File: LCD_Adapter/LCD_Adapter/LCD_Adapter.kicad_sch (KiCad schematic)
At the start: 2 parts, among them J1 2-1734248-0, J2 FH12-30S-0.5SH_55_

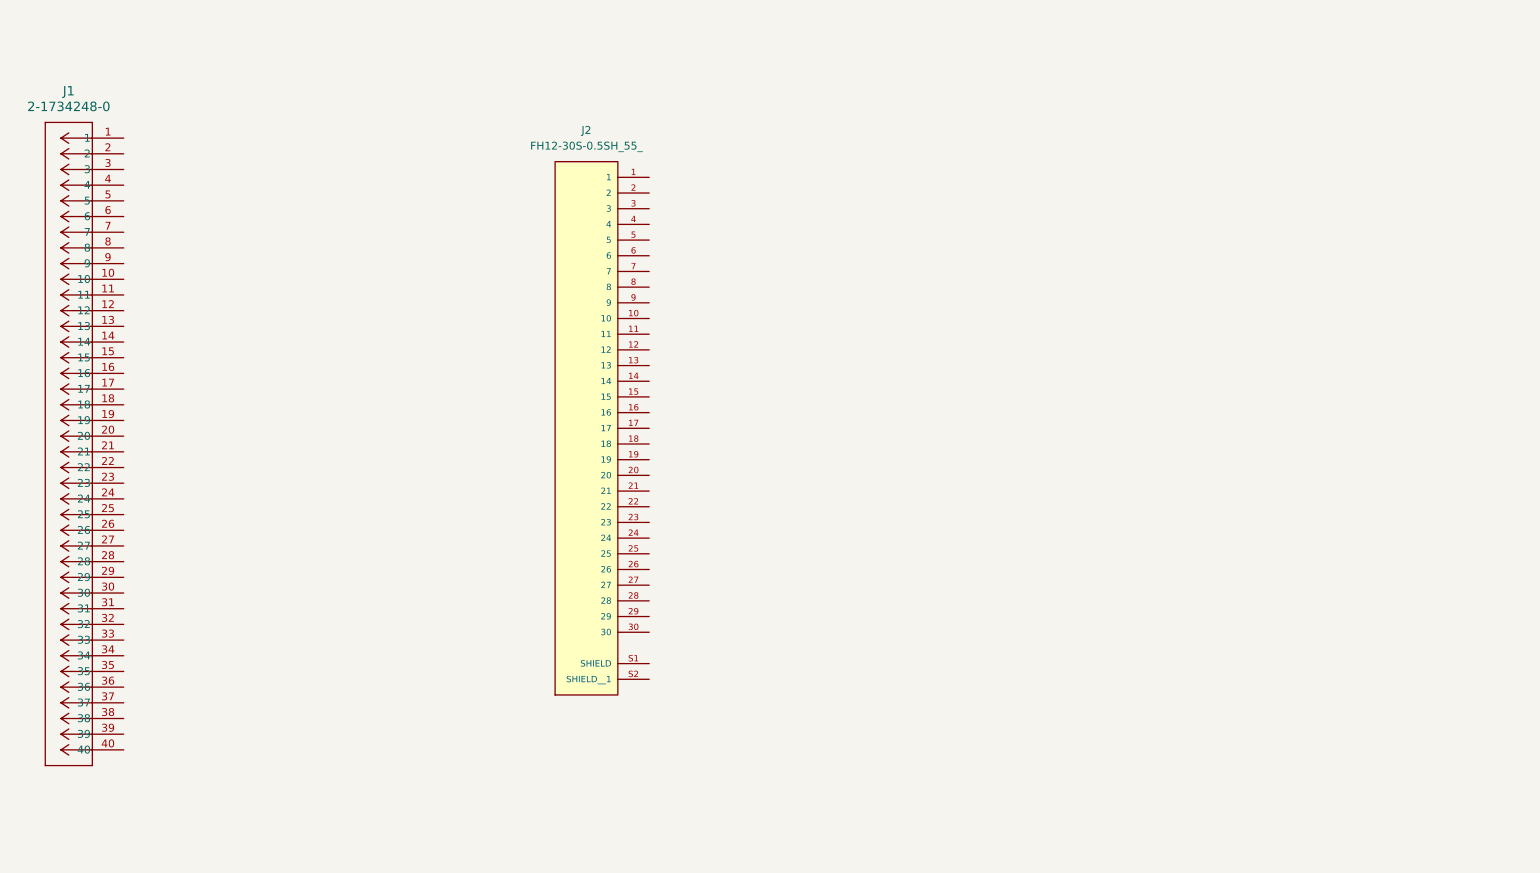
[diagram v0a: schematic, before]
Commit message: PSB_ADAPTER UPDATE
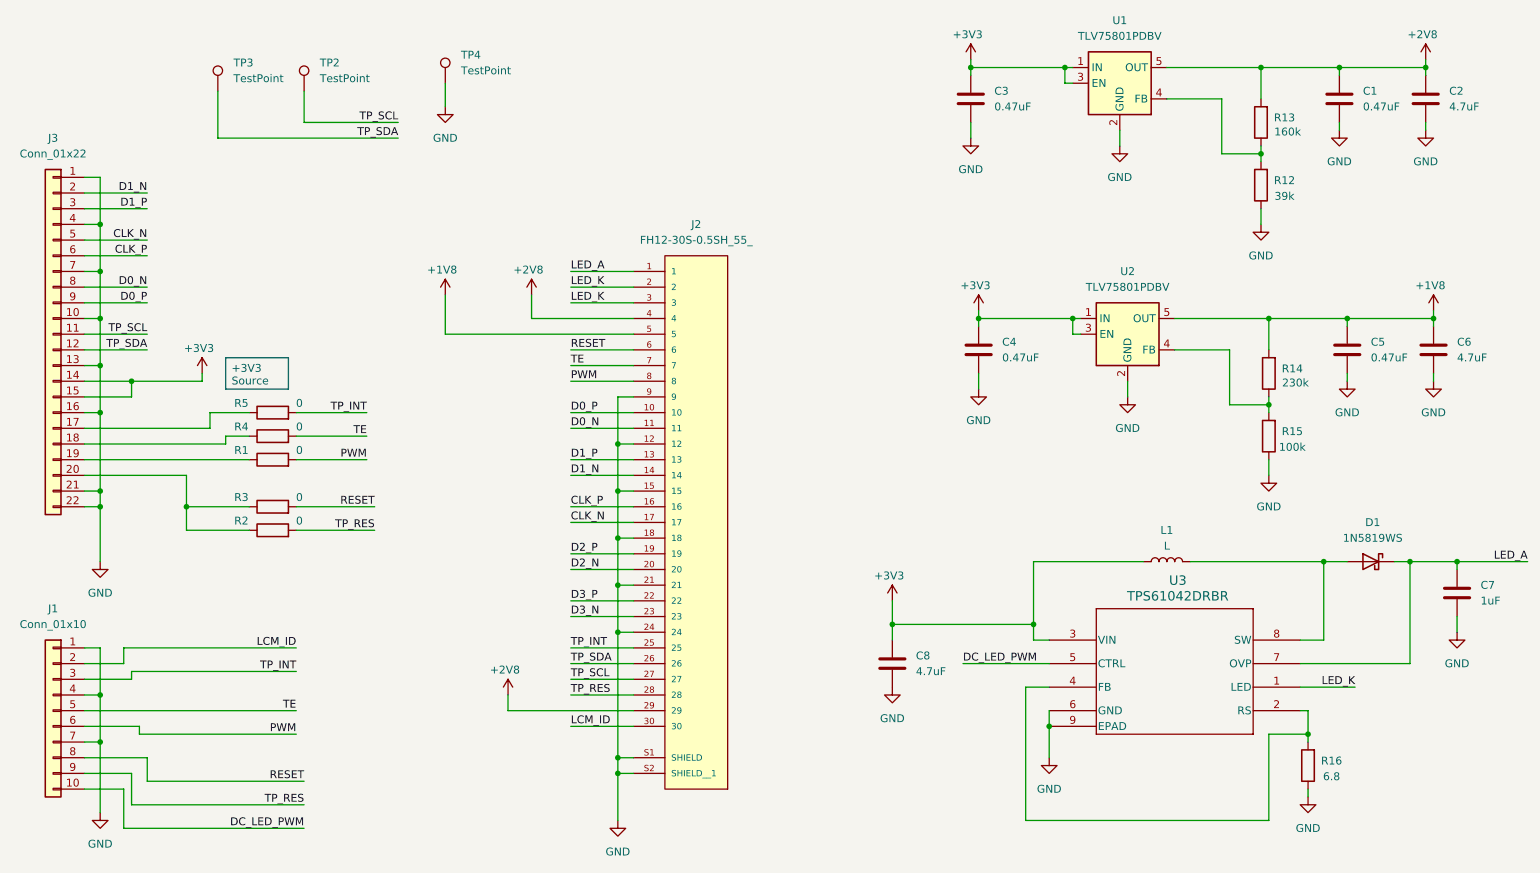
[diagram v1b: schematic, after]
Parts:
- removed J1: 2-1734248-0, lib:2-1734248-0, symbol 2-1734248-0:2-1734248-0
- added C1, C3, C4, C5: 0.47uF, Capacitor_SMD:C_0603_1608Metric, symbol Device:C
- added C2, C6, C8: 4.7uF, Capacitor_SMD:C_0603_1608Metric, symbol Device:C
- added C7: 1uF, Capacitor_SMD:C_0603_1608Metric, symbol Device:C
- added D1: 1N5819WS, Diode_SMD:D_SOD-323, symbol Diode:1N5819WS
- added J1: Conn_01x10, Connector_PinHeader_2.54mm:PinHeader_1x10_P2.54mm_Vertical, symbol Connector_Generic:Conn_01x10
- added J3: Conn_01x22, lib:FC-10A20P11H20, symbol Connector_Generic:Conn_01x22
- added L1: L, Inductor_SMD:L_1210_3225Metric, symbol Device:L
- added R1, R2, R3, R4, R5: 0, Resistor_SMD:R_0603_1608Metric, symbol Device:R
- added R12: 39k, Resistor_SMD:R_0603_1608Metric, symbol Device:R
- added R13: 160k, Resistor_SMD:R_0603_1608Metric, symbol Device:R
- added R14: 230k, Resistor_SMD:R_0603_1608Metric, symbol Device:R
- added R15: 100k, Resistor_SMD:R_0603_1608Metric, symbol Device:R
- added R16: 6.8, Resistor_SMD:R_0603_1608Metric, symbol Device:R
- added TP2, TP3, TP4: TestPoint, TestPoint:TestPoint_Pad_D1.0mm, symbol Connector:TestPoint
- added U1, U2: TLV75801PDBV, Package_TO_SOT_SMD:SOT-23-5, symbol Regulator_Linear:TLV75801PDBV
- added U3: TPS61042DRBR, lib:DRB8_1P75X1P5, symbol TPS61042:TPS61042DRBR
- J2: footprint FH12-30S-0.5SH_55_:HIROSE_FH12-30S-0.5SH_55_ -> lib:HIROSE_FH12-30S-0.5SH_55_
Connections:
- net  LED_A: now reaches J2.1
- net  LED_A: now also C7.1, D1.1 (K), U3.7 (OVP)
- net D0_P: now reaches J2.10
- net D0_P: now also J3.9 (Pin_9)
- net D0_N: now reaches J2.11
- net D0_N: now also J3.8 (Pin_8)
- net GND: now reaches J2.12
- net GND: now also J2.15, J2.18, J2.21, J2.24, J2.9, J2.S1 (SHIELD), J2.S2 (SHIELD__1), C1.2, C2.2, C3.2, C4.2, C5.2, C6.2, C7.2, C8.2, J1.1 (Pin_1), J1.4 (Pin_4), J1.7 (Pin_7), J3.1 (Pin_1), J3.10 (Pin_10), J3.13 (Pin_13), J3.16 (Pin_16), J3.21 (Pin_21), J3.22 (Pin_22), J3.4 (Pin_4), J3.7 (Pin_7), R12.1, R15.1, R16.1, TP4.1, U1.2 (GND), U2.2 (GND), U3.6 (GND), U3.9 (EPAD)
- net D1_P: now reaches J2.13
- net D1_P: now also J3.3 (Pin_3)
- net D1_N: now reaches J2.14
- net D1_N: now also J3.2 (Pin_2)
- net CLK_P: now reaches J2.16
- net CLK_P: now also J3.6 (Pin_6)
- net CLK_N: now reaches J2.17
- net CLK_N: now also J3.5 (Pin_5)
- net D2_P: now reaches J2.19
- net  LED_K: now reaches J2.2
- net  LED_K: now also J2.3, U3.1 (LED)
- net D2_N: now reaches J2.20
- net D3_P: now reaches J2.22
- net D3_N: now reaches J2.23
- net TP_INT: now reaches J2.25
- net TP_INT: now also J1.3 (Pin_3), R5.2
- net TP_SDA: now reaches J2.26
- net TP_SDA: now also J3.12 (Pin_12), TP3.1
- net TP_SCL: now reaches J2.27
- net TP_SCL: now also J3.11 (Pin_11), TP2.1
- net TP_RES: now reaches J2.28
- net TP_RES: now also J1.9 (Pin_9), R2.2
- net +2V8: now reaches J2.29
- net +2V8: now also J2.4, C1.1, C2.1, R13.2, U1.5 (OUT)
- net LCM_ID: now reaches J2.30
- net LCM_ID: now also J1.2 (Pin_2)
- net +1V8: now reaches J2.5
- net +1V8: now also C5.1, C6.1, R14.2, U2.5 (OUT)
- net RESET: now reaches J2.6
- net RESET: now also J1.8 (Pin_8), R3.2
- net TE: now reaches J2.7
- net TE: now also J1.5 (Pin_5), R4.2
- net PWM: now reaches J2.8
- net PWM: now also J1.6 (Pin_6), R1.2
- new net: J3.19 (Pin_19), R1.1
- new net: R16.2, U3.2 (RS), U3.4 (FB)
- new net: D1.2 (A), L1.2, U3.8 (SW)
- new net: R14.1, R15.2, U2.4 (FB)
- new net: J3.17 (Pin_17), R5.1
- new net: J3.18 (Pin_18), R4.1
- new net: J3.20 (Pin_20), R2.1, R3.1
- new net: R12.2, R13.1, U1.4 (FB)
- new net +3V3: C3.1, C4.1, C8.1, J3.14 (Pin_14), J3.15 (Pin_15), L1.1, U1.1 (IN), U1.3 (EN), U2.1 (IN), U2.3 (EN), U3.3 (VIN)
- new net DC_LED_PWM: J1.10 (Pin_10), U3.5 (CTRL)
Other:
- moved on the sheet: J2
